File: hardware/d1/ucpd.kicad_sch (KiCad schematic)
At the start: 41 parts, among them Q1 CSD17577Q3A, Q2 CSD17577Q3A, U15 ESDA25P35-1U1M, U16 ESDA25P35-1U1M, U4 TCPP03-M20, U5 TCPP03-M20

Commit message: Fixesss
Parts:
- USBC2: now left out of the parts list
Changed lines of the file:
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@@
 		(body_style 1)
 		(exclude_from_sim no)
-		(in_bom yes)
+		(in_bom no)
 		(on_board yes)
-		(in_pos_files yes)
+		(in_pos_files no)
 		(dnp no)
 		(fields_autoplaced yes)

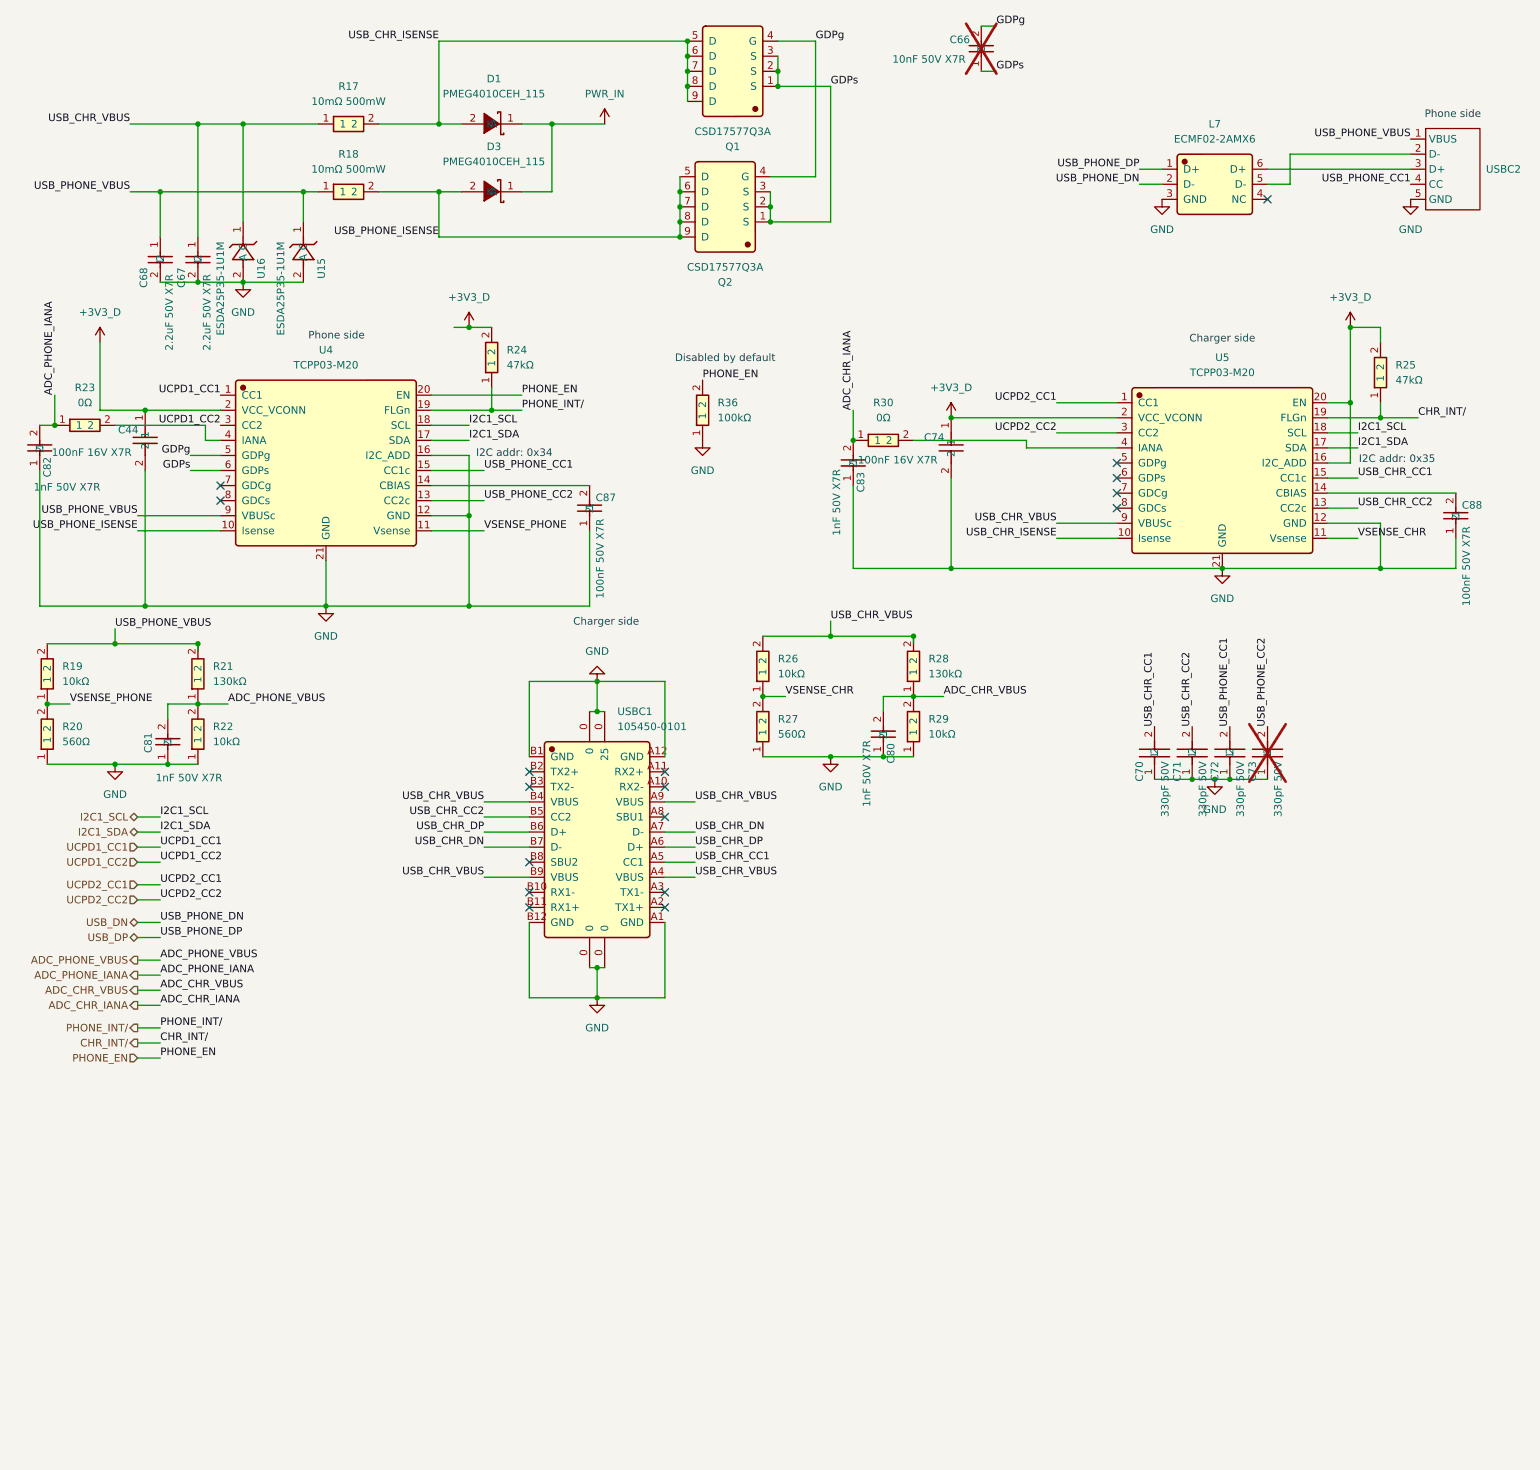
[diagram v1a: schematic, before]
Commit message: Fixes
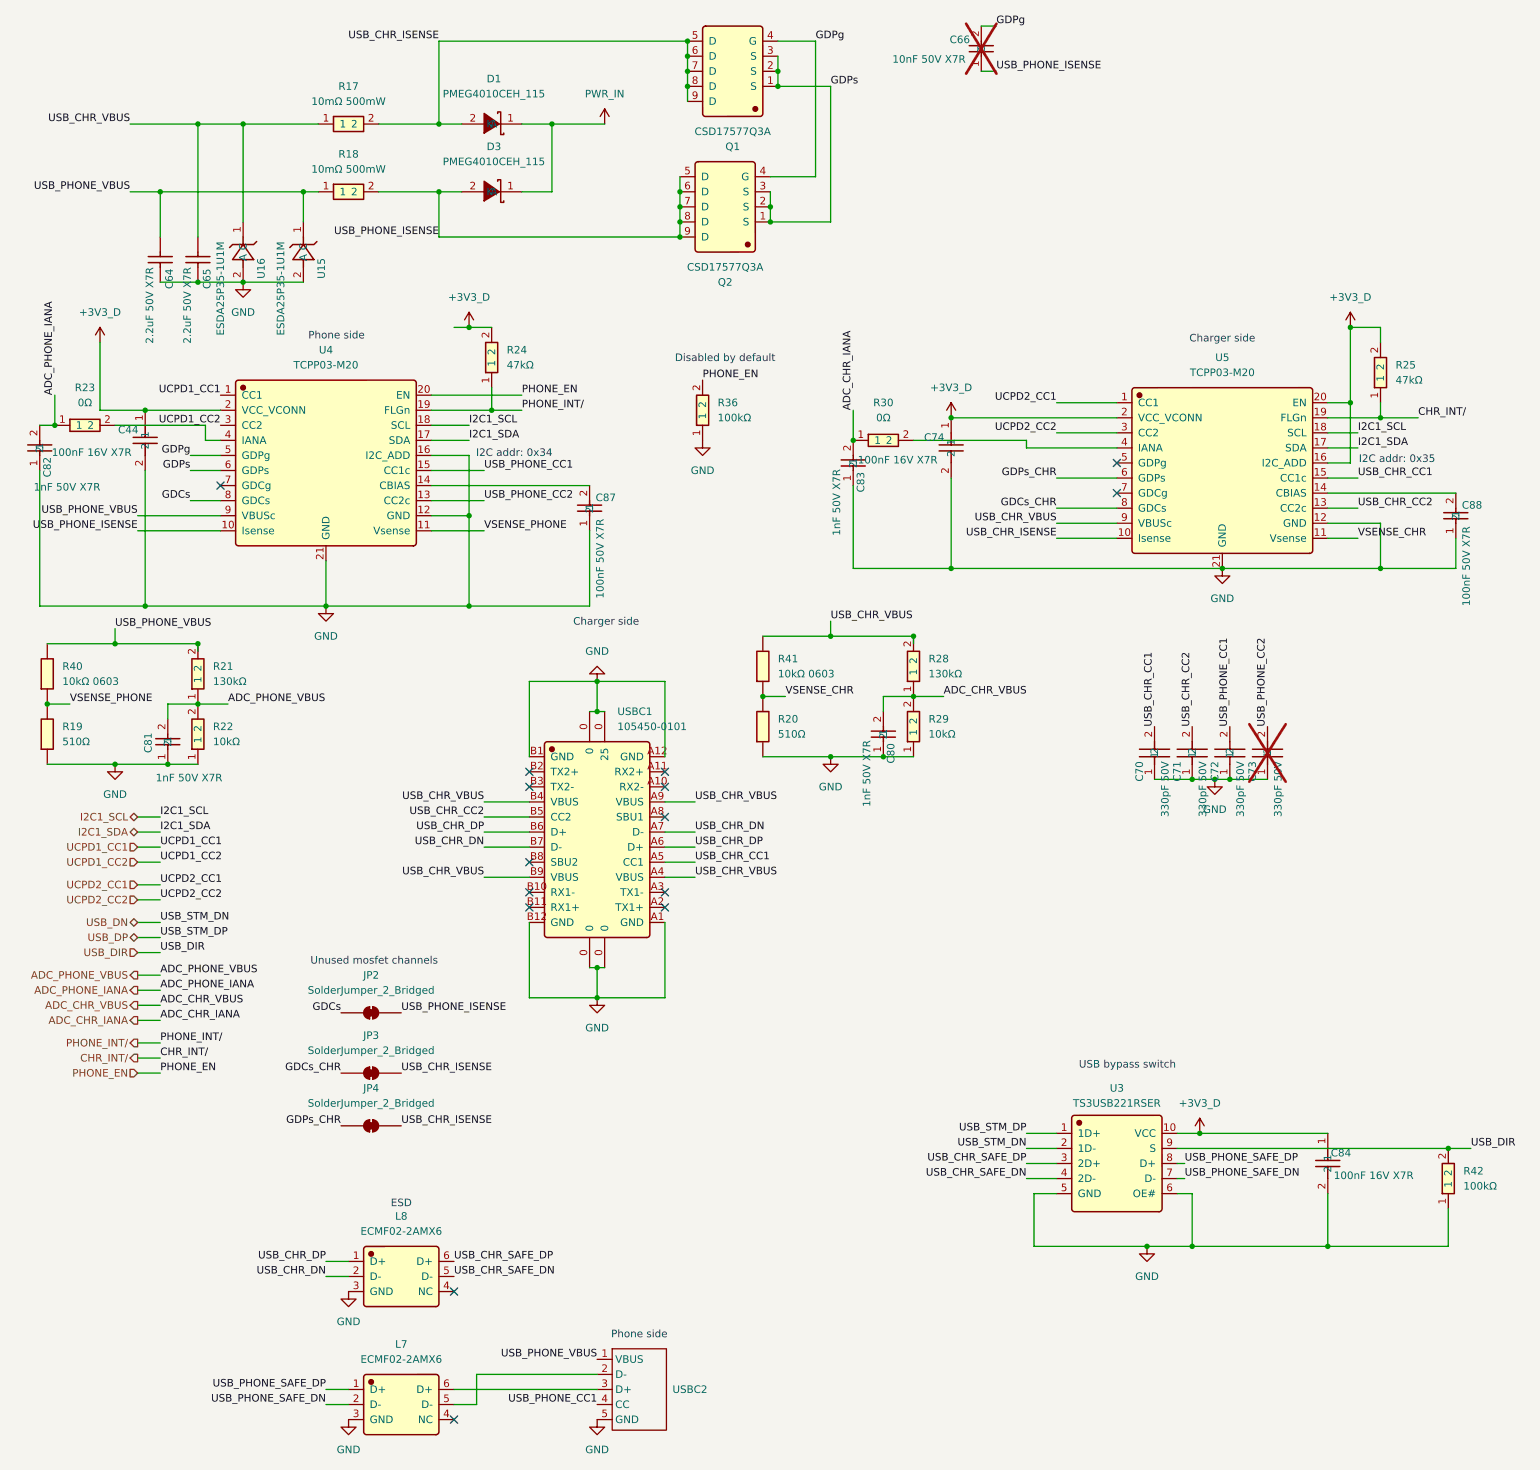
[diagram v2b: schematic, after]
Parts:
- removed C67, C68: 2.2uF 50V X7R, JLCImport:CC0805KKX7R9BB225, symbol JLCImport:CC0805KKX7R9BB225
- removed R19, R26: 10kΩ, Resistor_SMD:R_0402_1005Metric, symbol JLCImport:0402WGF1002TCE
- removed R20, R27: 560Ω, Resistor_SMD:R_0402_1005Metric, symbol JLCImport:0402WGF5600TCE
- added C64, C65: 2.2uF 50V X7R, Capacitor_SMD:C_1206_3216Metric, symbol JLCImport:CL31B225KBHNNNE
- added C84: 100nF 16V X7R, JLCImport:CL05B104KO5NNNC, symbol JLCImport:CL05B104KO5NNNC
- added JP2, JP3, JP4: SolderJumper_2_Bridged, Jumper:SolderJumper-2_P1.3mm_Bridged_RoundedPad1.0x1.5mm, symbol Jumper:SolderJumper_2_Bridged
- added L8: ECMF02-2AMX6, JLCImport:ECMF02-2AMX6, symbol JLCImport:ECMF02-2AMX6
- added R19, R20: 510Ω, Resistor_SMD:R_0603_1608Metric, symbol JLCImport:0603WAJ0511T5E
- added R40, R41: 10kΩ 0603, Resistor_SMD:R_0603_1608Metric, symbol JLCImport:RC0603FR-0710KL
- added R42: 100kΩ, JLCImport:0402WGF1003TCE, symbol JLCImport:0402WGF1003TCE
- added U3: TS3USB221RSER, JLCImport:TS3USB221RSER, symbol JLCImport:TS3USB221RSER
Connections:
- net +3V3_D: now also C84.1, U3.10 (VCC)
- net GDPs: no longer C66.1
- net GND: now also C64.1, C65.1, C84.2, L8.3 (GND), R19.1, R20.1, R42.1, U3.5 (GND), U3.6 (OE#)
- net USB_CHR_DN: now also L8.2 (D-)
- net USB_CHR_DP: now also L8.1 (D+)
- net USB_CHR_ISENSE: now also JP3.2 (B), JP4.2 (B)
- net USB_CHR_VBUS: now also C65.2, R41.2
- net USB_DN: now also U3.2 (1D-); no longer L7.2 (D-)
- net USB_DP: now also U3.1 (1D+); no longer L7.1 (D+)
- net USB_PHONE_ISENSE: now also C66.1, JP2.2 (B)
- net USB_PHONE_VBUS: now also C64.2, R40.2
- net VSENSE_CHR: now also R20.2, R41.1
- net VSENSE_PHONE: now also R19.2, R40.1
- net GDPs_CHR: now reaches U5.6 (GDPs)
- net GDPs_CHR: now also JP4.1 (A)
- net GDCs_CHR: now reaches U5.8 (GDCs)
- net GDCs_CHR: now also JP3.1 (A)
- net GDCs: now reaches U4.8 (GDCs)
- net GDCs: now also JP2.1 (A)
- new net USB_CHR_SAFE_DN: L8.5 (D-), U3.4 (2D-)
- new net USB_CHR_SAFE_DP: L8.6 (D+), U3.3 (2D+)
- new net USB_DIR: R42.2, U3.9 (S)
- new net USB_PHONE_SAFE_DN: L7.2 (D-), U3.7 (D-)
- new net USB_PHONE_SAFE_DP: L7.1 (D+), U3.8 (D+)
- no-connect marks 17 -> 15
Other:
- note added: "ESD"
- note added: "USB bypass switch"
- note added: "Unused mosfet channels"
- moved on the sheet: L7, USBC2
